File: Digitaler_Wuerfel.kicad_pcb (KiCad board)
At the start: 2 copper layers, 69.5 x 90.5 mm, 53 parts, among them J1 Conn_02x03_Odd_Even, J2 Conn_01x03_Pin, Q1 2N3904, SW1 SW_Push, SW2 SW_Push, SW3 SW_Push, SW4 SW_SPST, U1 MAX2650EUS+T, U2 MAX2650EUS+T, U3 74HC595, U4 74HC595, U5 MIC5219-5.0YM5, U6 ATmega328PB-A

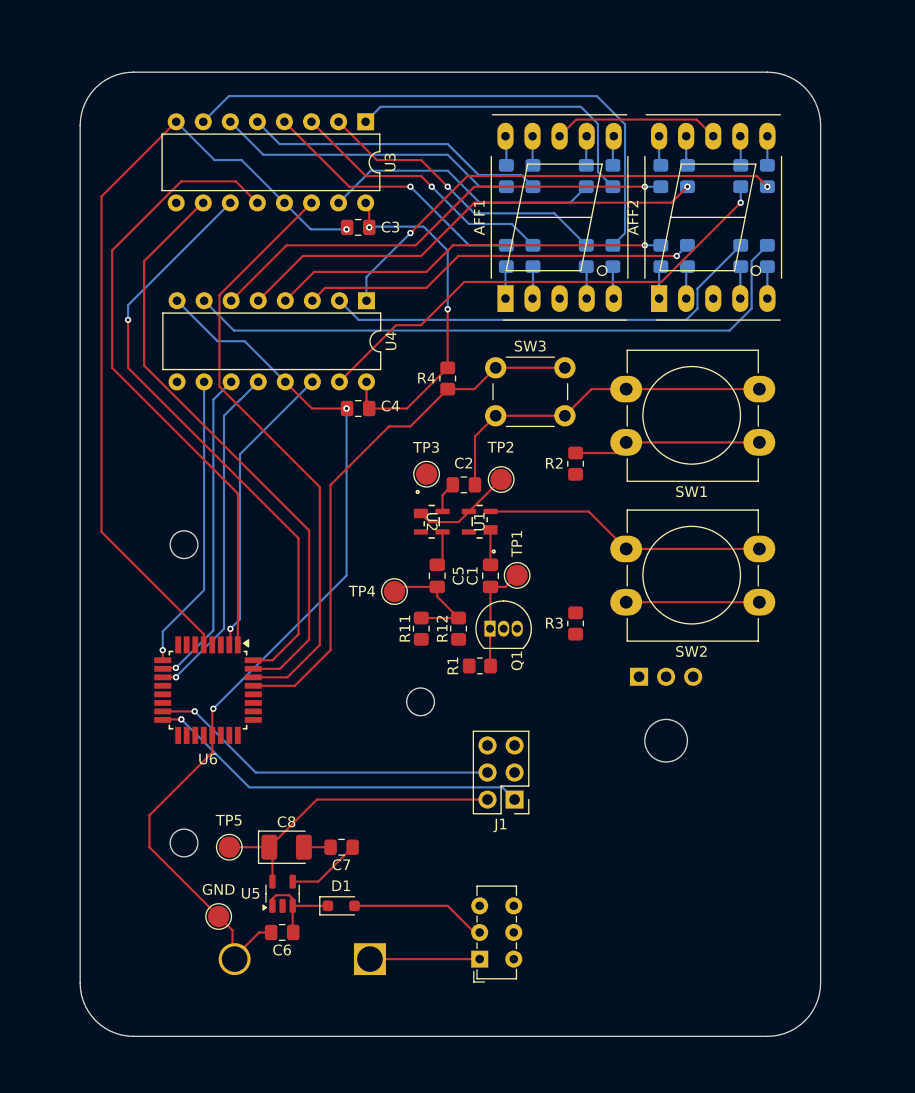
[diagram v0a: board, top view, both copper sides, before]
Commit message: Finished tracing
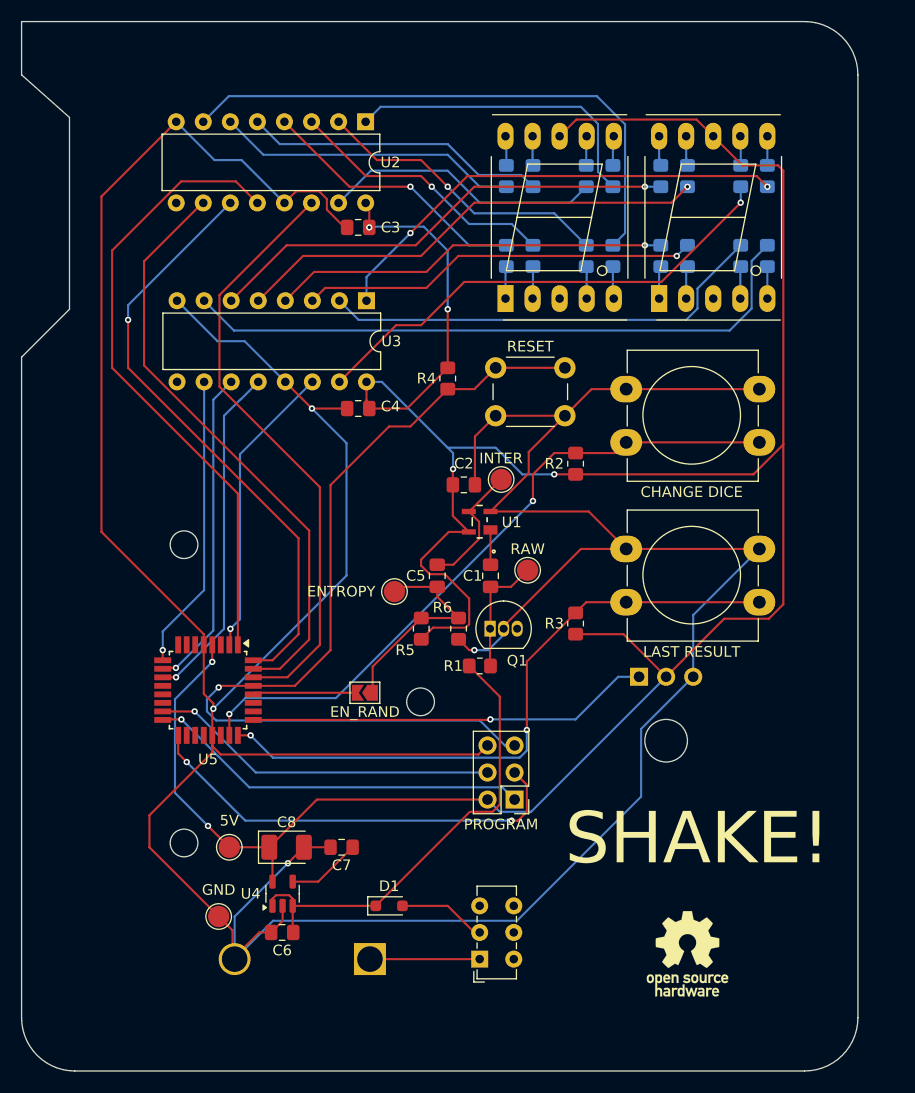
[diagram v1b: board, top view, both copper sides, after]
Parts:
- removed TP3: TestPoint_Probe, TestPoint:TestPoint_Pad_D2.0mm
- removed the U2 at (109.0, 68.4)
- added EN_RAND: SolderJumper_2_Open, Jumper:SolderJumper-2_P1.3mm_Open_TrianglePad1.0x1.5mm, F.Cu at (102.7, 84.5)
- added REF**: OSHW-Logo_7.5x8mm_SilkScreen, Symbol:OSHW-Logo_7.5x8mm_SilkScreen, F.Cu at (133.0, 109.0)
- CHANGE DICE: renamed from SW1
- LAST RESULT: renamed from SW2
- moved D1 4.50 mm to (105.0, 104.5)
- moved RAW 1.10 mm to (118.0, 73.0)
- renumbered TP5 to 5V, TP4 to ENTROPY, TP2 to INTER, J1 to PROGRAM, R8 to R10, R9 to R11, R10 to R12, R11 to R5, R12 to R6, R5 to R7, R6 to R8, R7 to R9, TP1 to RAW, SW3 to RESET, U3 to U2, U4 to U3, U5 to U4, U6 to U5
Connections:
- BT1 pad 1: +9V -> Net-(BT1-+)
- C5 pad 1: Net-(U2-OUT) -> Net-(U1-OUT)
- C5 pad 2: ENTROPY -> Net-(JP1-A)
- C6 pad 1: Net-(D1-K) -> +9V
- D1 pad 1: Net-(D1-K) -> +9V
- ENTROPY pad 1: ENTROPY -> Net-(JP1-A)
- R5 pad 2: ENTROPY -> Net-(JP1-A)
- R6 pad 1: ENTROPY -> Net-(JP1-A)
- SW4 pad 1: +9V -> Net-(BT1-+)
- SW4 pad 4: +9V -> (no net)
- SW4 pad 5: Net-(D1-A) -> (no net)
- U4 pad 1: Net-(D1-K) -> +9V
- U4 pad 3: Net-(D1-K) -> +9V
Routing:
- net +5V: track 81.4 -> 268.2 mm, vias 2 -> 6
- net GND: track 225.8 -> 383.4 mm, vias 3 -> 4
- net BTN_LAST: track 12.5 -> 60.8 mm, vias 0 -> 2
- net BTN_CH: track 17.7 -> 63.8 mm, vias 0 -> 2
- net SPI_CLK: track 0.00 -> 41.5 mm, vias 0 -> 2
- net SHAKE_OUT: track 0.00 -> 37.9 mm, vias 0 -> 1
- net RESET: track 50.7 -> 86.9 mm, vias 0 -> 1
- net +9V: track 10.5 -> 43.6 mm
- net Net-(JP1-A): track 0.00 -> 20.4 mm
- net Net-(BT1-+): track 0.00 -> 10.5 mm
- net Net-(D1-K): track 9.33 -> 0.00 mm
- net Net-(D1-A): track 12.8 -> 8.29 mm
- net Net-(U2-OUT): track 3.29 -> 0.00 mm
- net Net-(U1-OUT): track 9.54 -> 12.2 mm
- net ENTROPY: track 11.5 -> 9.81 mm
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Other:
- board size 69.5 x 90.5 mm -> 78.5 x 98.5 mm
- board text added: "SHAKE!"
- board text added: "by Jan Wielpütz https://github.com/janWie96/SchuettelDice.git"
